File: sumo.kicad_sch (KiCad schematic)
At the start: 55 parts, among them Q1 BPW40, Q2 BPW40, SW1 SW_Push, SW2 SW_DIP_x01, SW3 SW_DIP_x01, SW4 SW_DIP_x01, T1 Screw_Terminal_01x04, T2 Screw_Terminal_01x04, T3 Screw_Terminal_01x04, T4 Screw_Terminal_01x04, T5 Screw_Terminal_01x04, U1 PIC16F628A-IP, U2 L7805, U3 L293D, U4 74HC04, U5 TSOP4038, U6 TSOP4038

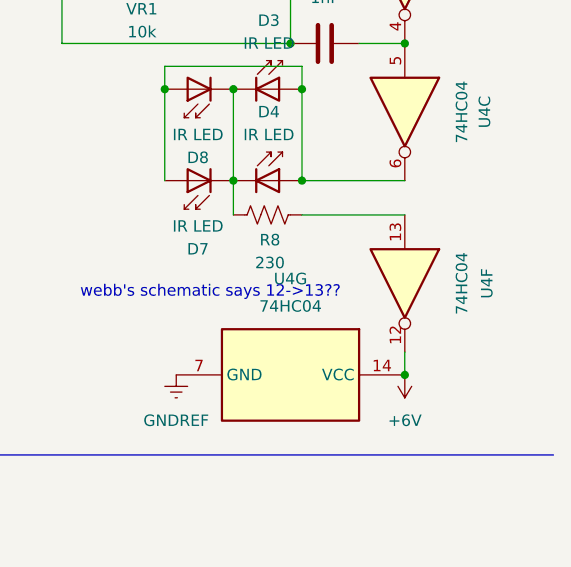
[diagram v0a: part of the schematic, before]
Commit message: sensors
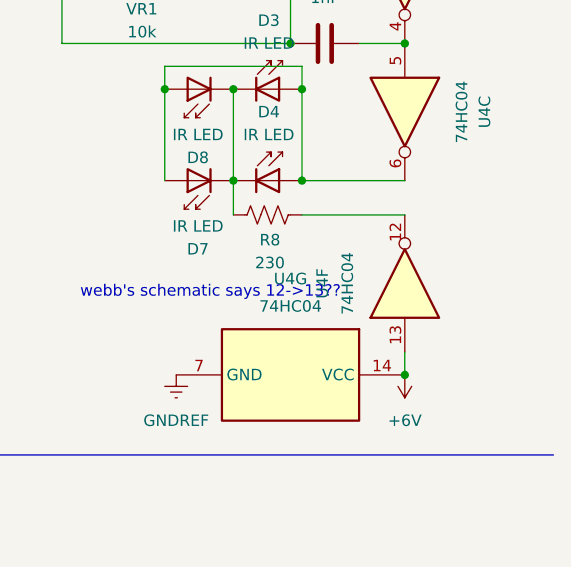
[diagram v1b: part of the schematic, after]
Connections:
- net +6V: now also U4.13; no longer U4.12
- net at R8.2: now also U4.12; no longer U4.13
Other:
- moved on the sheet: U4F
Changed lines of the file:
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@@
 	(symbol
 		(lib_id "74xx:74HC04")
-		(at 267.97 83.82 270)
+		(at 267.97 83.82 90)
 		(unit 6)
 		(exclude_from_sim no)
@@
 		(dnp no)
 		(property "Reference" "U4"
-			(at 277.114 83.82 0)
+			(at 258.826 83.82 0)
 			(effects
 				(font
@@
 		)
 		(property "Value" "74HC04"
-			(at 274.32 83.82 0)
+			(at 261.62 83.82 0)
 			(effects
 				(font

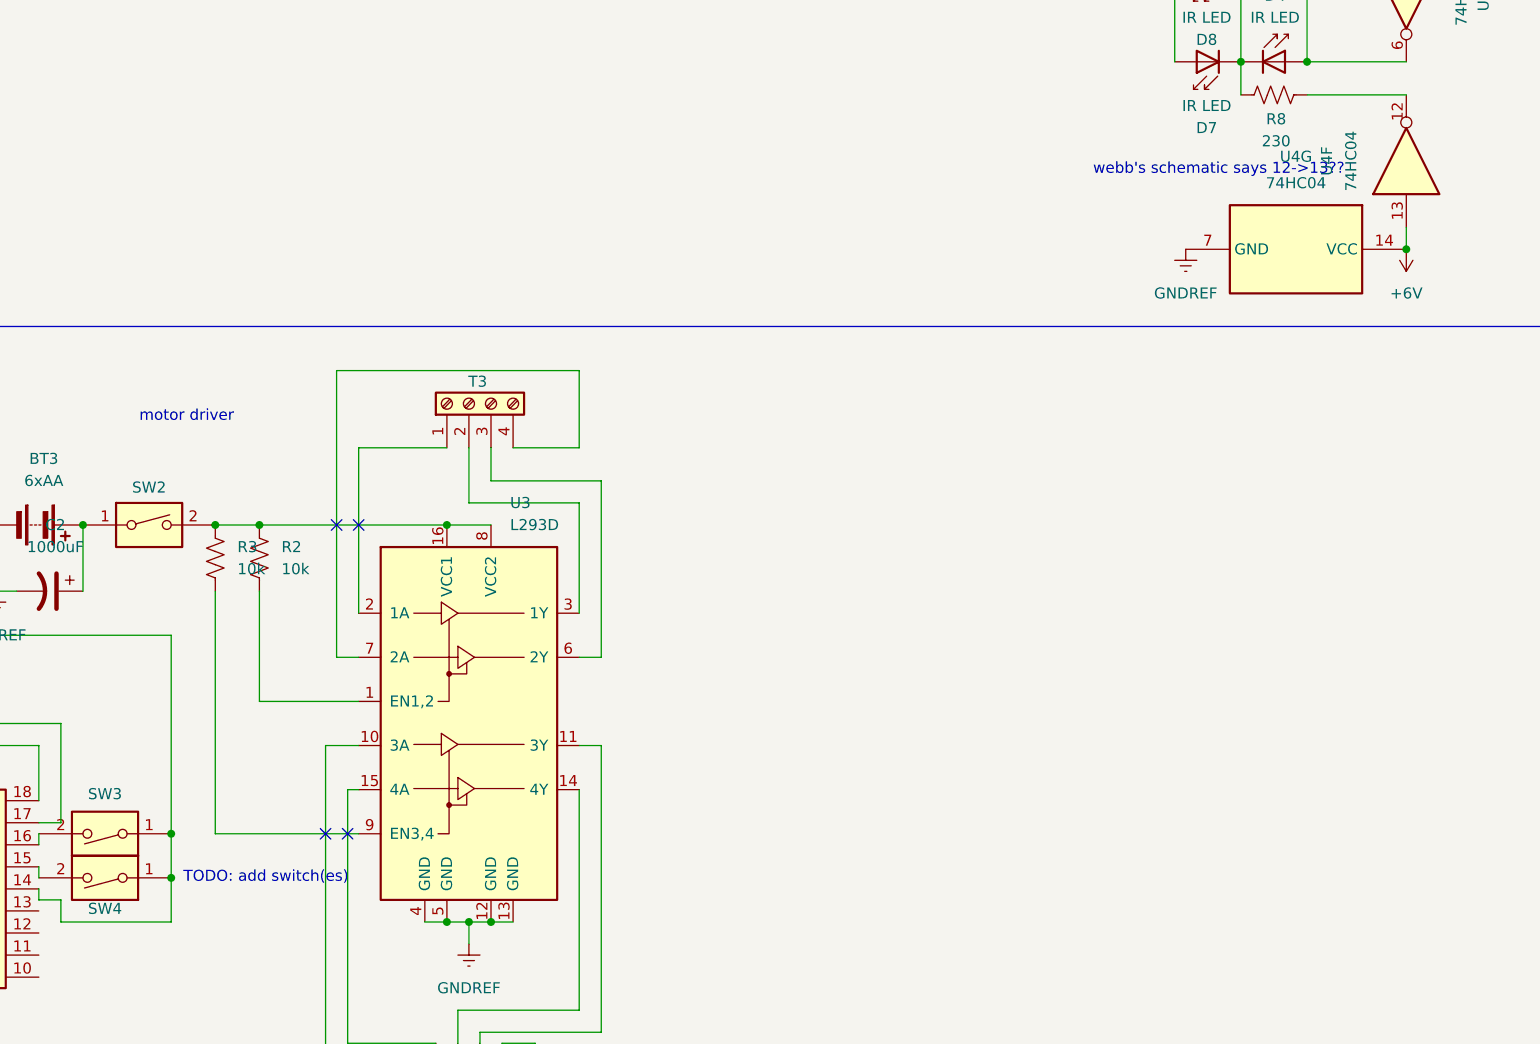
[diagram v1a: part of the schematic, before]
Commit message: save changes
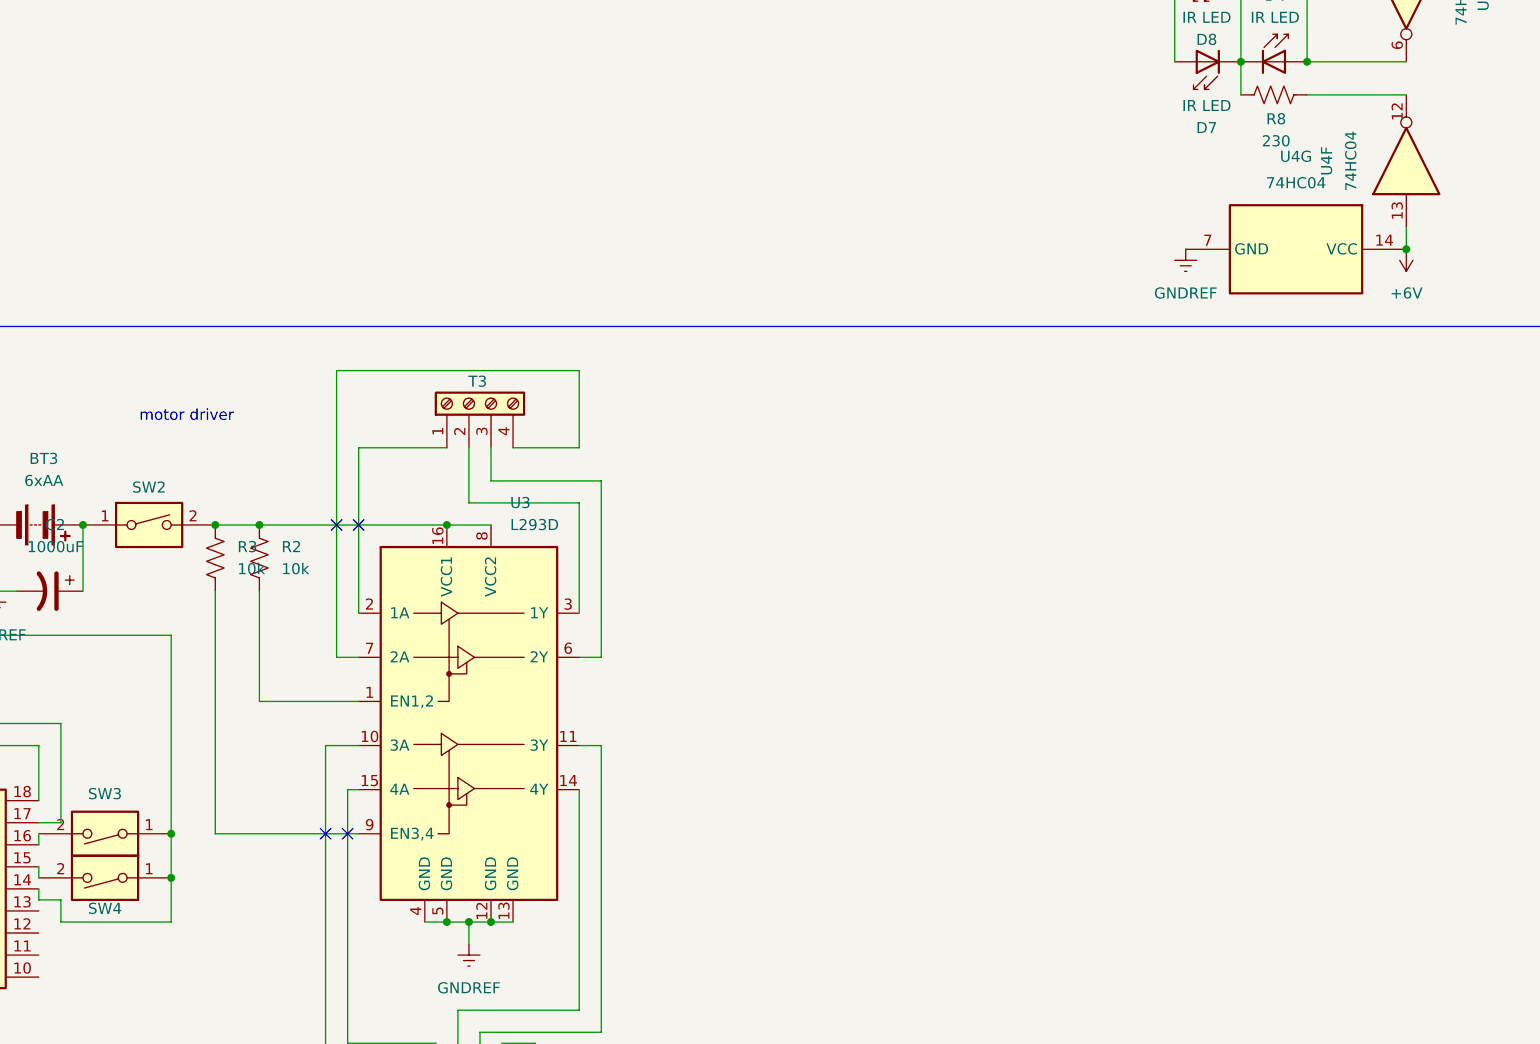
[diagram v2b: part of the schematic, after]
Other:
- note removed: "TODO: add switch(es)"
- note removed: "webb's schematic says 12->13??"
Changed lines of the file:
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@@
-		)
-	)
-	(text "webb's schematic says 12->13??\n"
-		(exclude_from_sim no)
-		(at 246.38 84.836 0)
-		(effects
-			(font
-				(size 1.27 1.27)
-			)
 		)
 	)
@@
 		(effects
 			(font
-				(size 1.27 1.27)
-			)
-		)
-	)
-	(text "TODO: add switch(es)"
-		(exclude_from_sim no)
-		(at 136.652 166.37 0)
-		(effects
-			(font
